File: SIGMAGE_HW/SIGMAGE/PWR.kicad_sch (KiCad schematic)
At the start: 44 parts, among them J18 HTSW10107GD, J19 HTSW10107GD, J22 HTSW10107GD, J23 HTSW10107GD, U1 MAX8902BATA/V+T, U11 TPS62130RGTT, U12 TPS62130RGTT, U2 MAX8902BATA/V+T

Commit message: almost done
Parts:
- added C14, C144, C16: 10u, Capacitor_SMD:C_0603_1608Metric, symbol Device:C
- added C143, C188: 1u, Capacitor_SMD:C_0603_1608Metric, symbol Device:C
- added C15: 10n, Capacitor_SMD:C_0603_1608Metric, symbol Device:C
- added C177: 100n, Capacitor_SMD:C_0603_1608Metric, symbol Device:C
- added C178: 3300p, Capacitor_SMD:C_0603_1608Metric, symbol Device:C
- added C187: 22u, Capacitor_SMD:C_0603_1608Metric, symbol Device:C
- added FB8, FB9: 500 @ 100 MHz, Capacitor_SMD:C_0603_1608Metric, symbol Device:FerriteBead
- added J26, J27: HTSW10107GD, SIGMAGE:HTSW10107GD, symbol SIGMAGE:HTSW10107GD
- added L3: 2200n XFL4020-222MEB, symbol Device:L
- added R112: 100k, Resistor_SMD:R_0603_1608Metric, symbol Device:R
- added R154: 60k, Resistor_SMD:R_0603_1608Metric, symbol Device:R
- added R155, R58: 120k, Resistor_SMD:R_0603_1608Metric, symbol Device:R
- added R3, R6: 440k, Resistor_SMD:R_0603_1608Metric, symbol Device:R
- added U31: MAX8902BATA/V+T, SIGMAGE:MAX8902BATAVT, symbol SIGMAGE:MAX8902BATAVT
- added U42: TPS62130RGTT, SIGMAGE:TPS62130RGTT, symbol SIGMAGE:TPS62130RGTT
- R24: value 60k -> 255k
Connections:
- net DVCC_1V2: now also J27.1; no longer J23.1
- net GND: now also C14.2, C143.2, C144.2, C16.2, C177.2, C178.2, C187.2, C188.2, R155.2, R58.2, U31.2 (GND), U31.4 (GS), U31.9 (EPAD), U42.15 (PGND), U42.16 (PGND), U42.17 (EPAD), U42.6 (AGND), U42.7 (FSW), U42.8 (DEF)
- net VCC_5V: now also C14.1, C144.1, C177.1, U31.1 (IN), U31.3 (EN), U42.10 (AVIN), U42.11 (PVIN), U42.12 (PVIN), U42.13 (EN)
- new net: C187.1, FB9.1, L3.2, R112.1, R154.1, U42.14 (VOS)
- new net: R154.2, R155.1, U42.5 (FB)
- new net: R3.2, R6.1
- new net: R58.1, R6.2, U31.6 (FB)
- new net: C188.1, FB9.2, J27.2
- new net: C15.1, C16.1, FB8.1, R3.1, U31.8 (OUT)
- new net: L3.1, U42.1 (SW), U42.2 (SW), U42.3 (SW)
- new net: R112.2, U42.4 (PG)
- new net: C178.1, U42.9 (SS/TR)
- new net: C143.1, FB8.2, J26.2
- new net: C15.2, U31.7 (BYP)
- new net AVCC_5V: J26.1
- new net DVCC_2V5: J23.1
- no-connect marks 2 -> 3
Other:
- moved on the sheet: C1, C2, C28, C29, C3, C30, C31, C32, C4, C5, C56, C57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

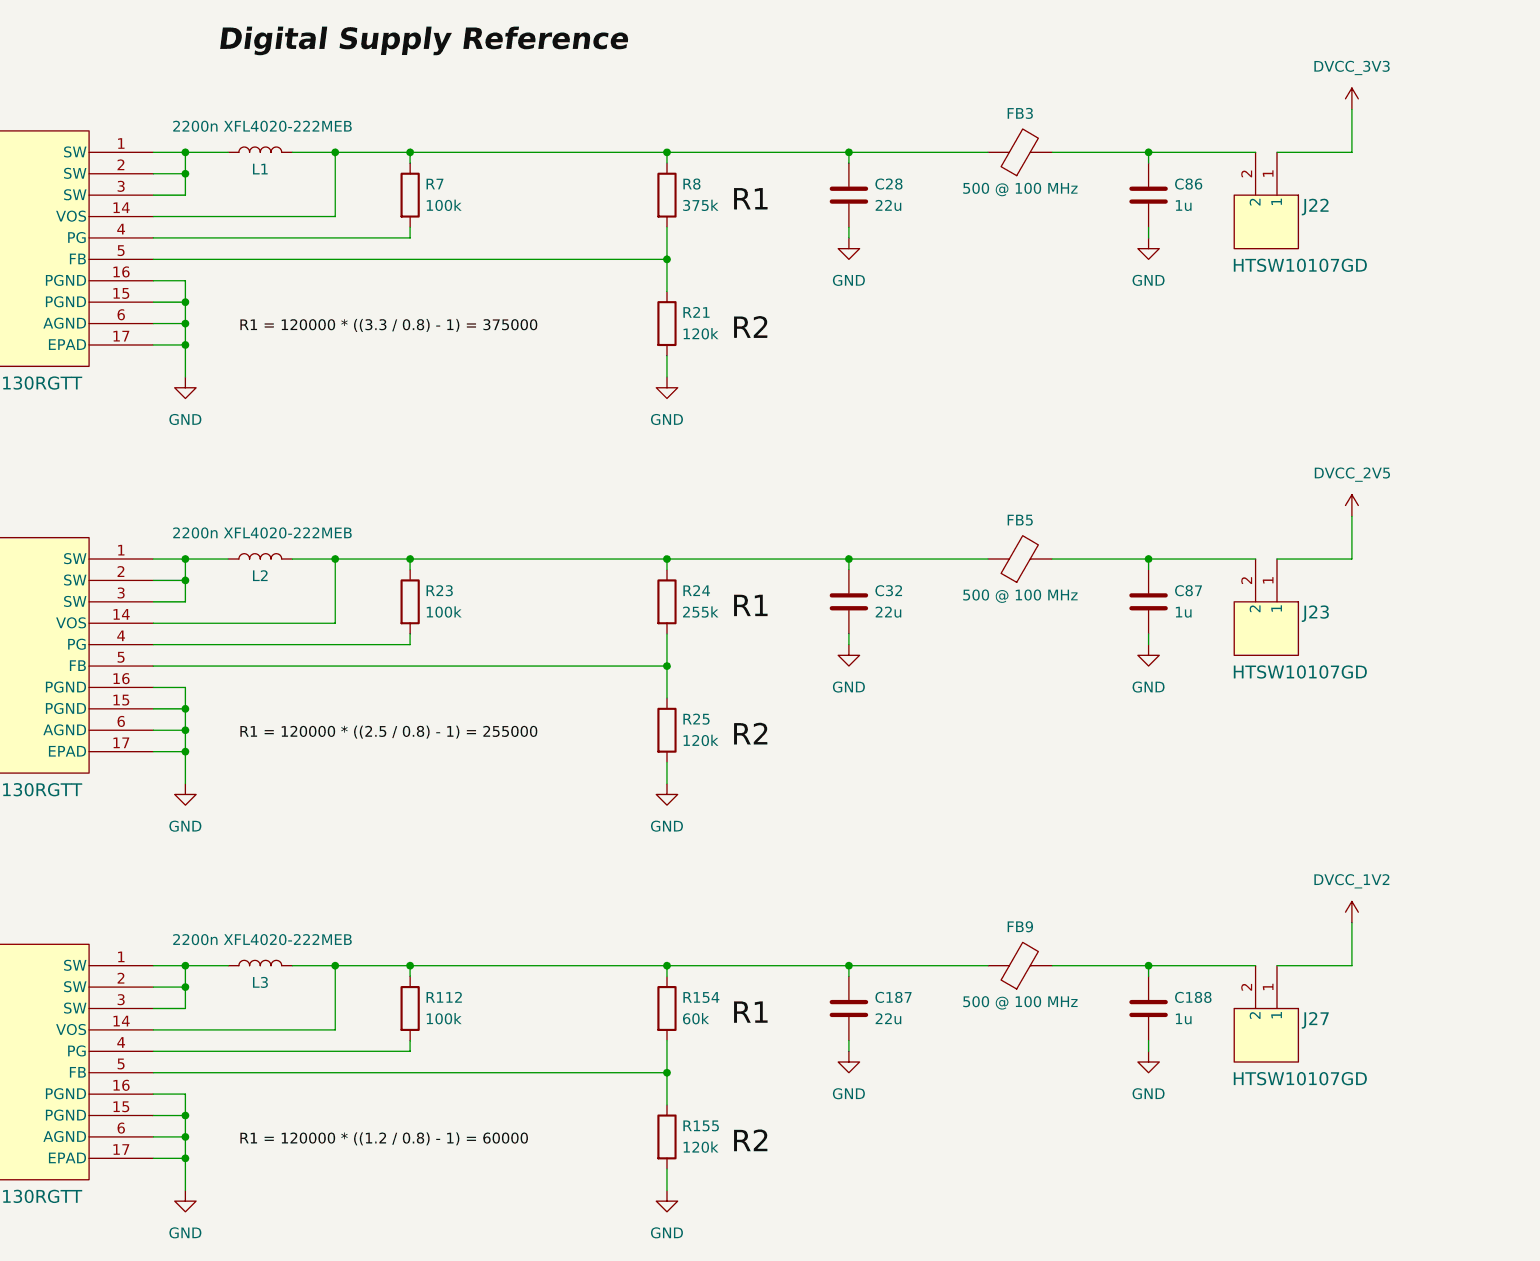
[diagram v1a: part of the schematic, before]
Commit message: some changes
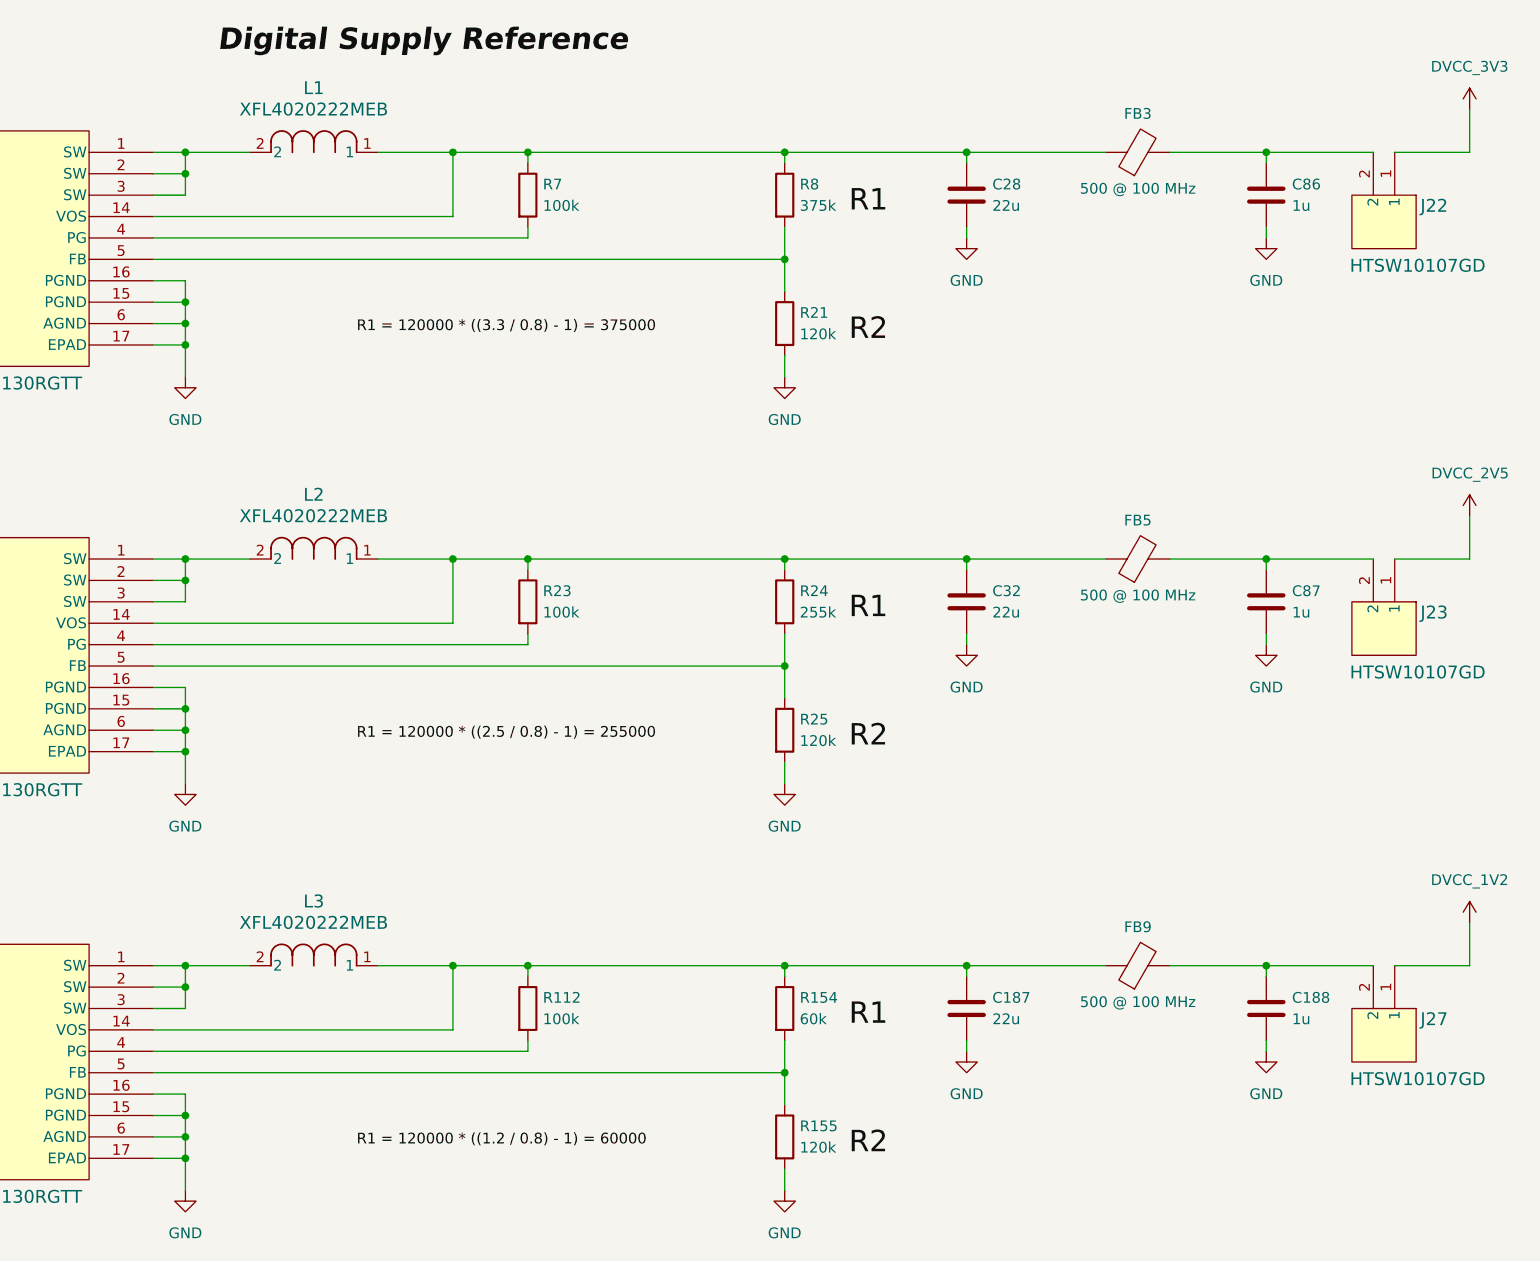
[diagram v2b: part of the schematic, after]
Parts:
- removed L1, L2, L3: 2200n XFL4020-222MEB, symbol Device:L
- added L1, L2, L3: XFL4020222MEB, SIGMAGE:XFL4020222MEB, symbol SIGMAGE:XFL4020222MEB
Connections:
- net at U12.1 (SW), U12.2 (SW), U12.3 (SW): now also L2.2
- net at C32.1, FB5.1, R23.1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: now also L2.1
- net at C187.1, FB9.1, R112.1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: now also L3.1
- net at U11.1 (SW), U11.2 (SW), U11.3 (SW): now also L1.2
- net at C28.1, FB3.1, R7.1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: now also L1.1
- net at U42.1 (SW), U42.2 (SW), U42.3 (SW): now also L3.2
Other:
- moved on the sheet: C187, C188, C28, C32, C86, C87, FB3, FB5, FB9, J22, J23, J27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
